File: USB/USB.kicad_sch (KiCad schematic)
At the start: 19 parts, among them J1 USBC-4-0-CX90MW9-24P1, U1 ESDA25L, U14 MUX HD3SS460RHRR, U15 USB SWITCH 2CHANNEL TS3USB221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, U16 usb-polarity-TUSB321RWBR

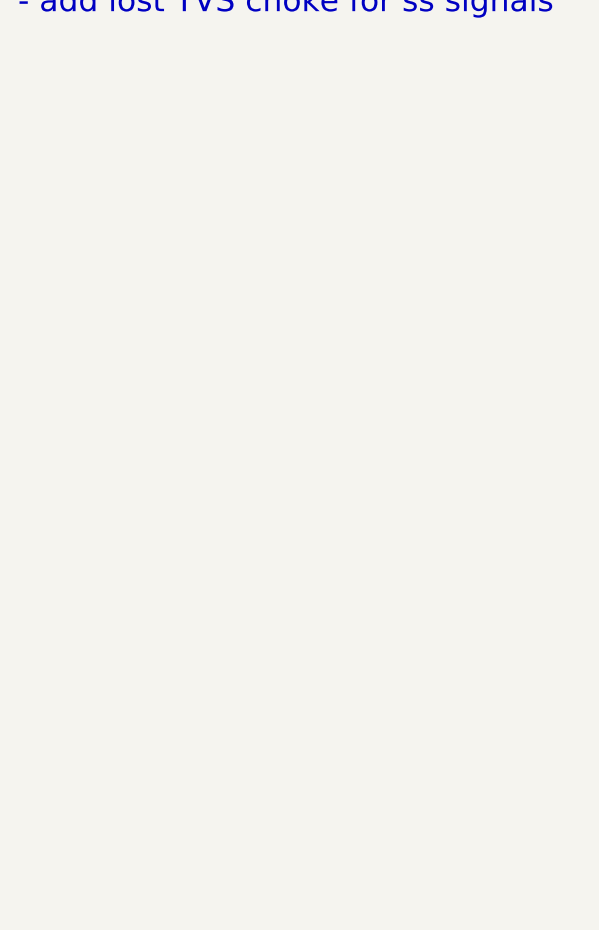
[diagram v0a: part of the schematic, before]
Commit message: add MPNs and datasheet
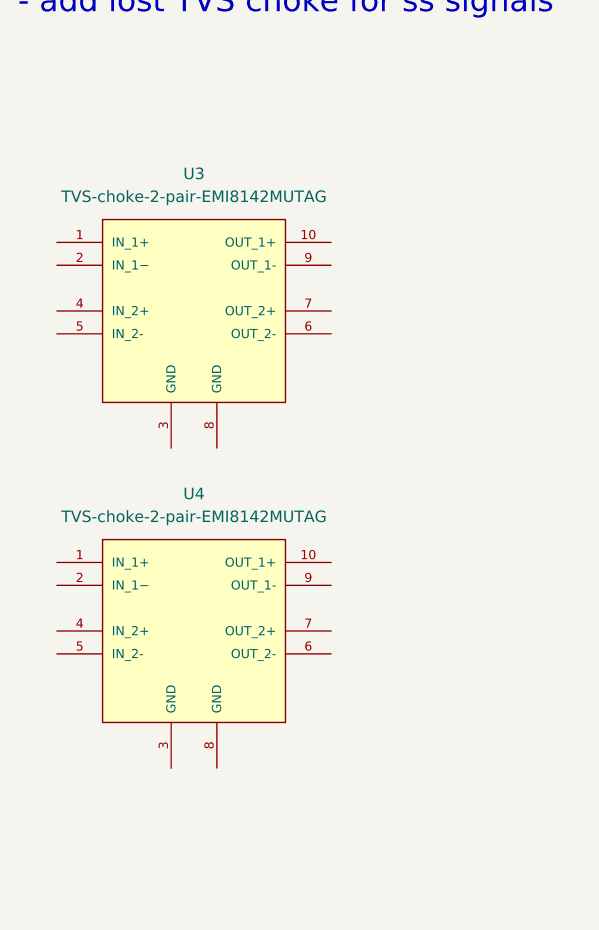
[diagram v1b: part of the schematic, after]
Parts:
- removed U2: ~, SPIRIT-footprints:1-line-tvs-choke-XDFN6, symbol SPIRIT-components:TVS-choke-1-lineEMI8141
- added U2: ~, SPIRIT-footprints:1-channel-TVS-choke-XDFN6_1P2X1P2_ONS, symbol SPIRIT-components:TVS-choke-1-pair-EMI8141
- added U3, U4: TVS-choke-2-pair-EMI8142MUTAG, SPIRIT-footprints:2-channel-TVS-chokeXDFN10_2P2X1P3_ONS, symbol SPIRIT-components:TVS-choke-2-pair-EMI8142MUTAG
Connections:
- net D+: now also U2.1 (D+IN)
- net D+f: now also U2.6 (D+OUT)
- net D-: now also U2.2 (D-IN)
- net D-f: now also U2.5 (D-OUT)
- net GND: now also U2.3 (GND), U2.4 (GND)
